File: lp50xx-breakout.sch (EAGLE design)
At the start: 17 parts, among them U1 LP5024

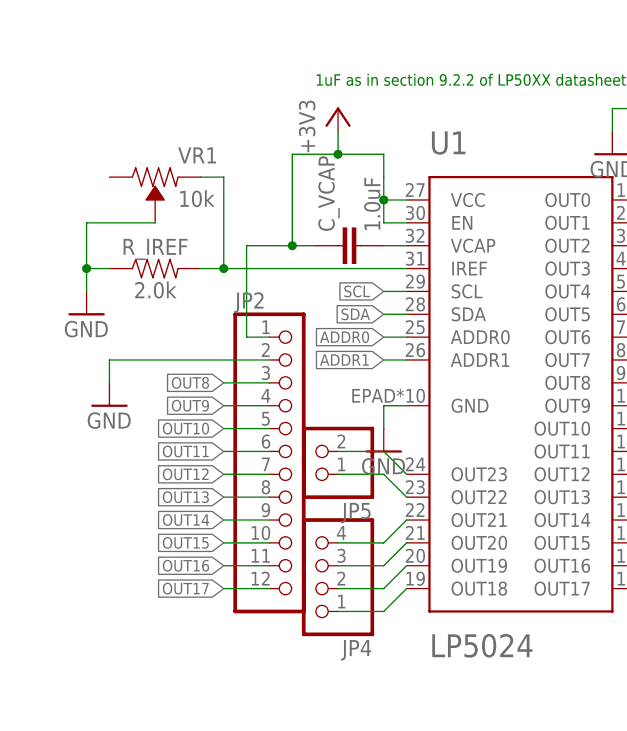
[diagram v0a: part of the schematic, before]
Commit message: Minor improvements
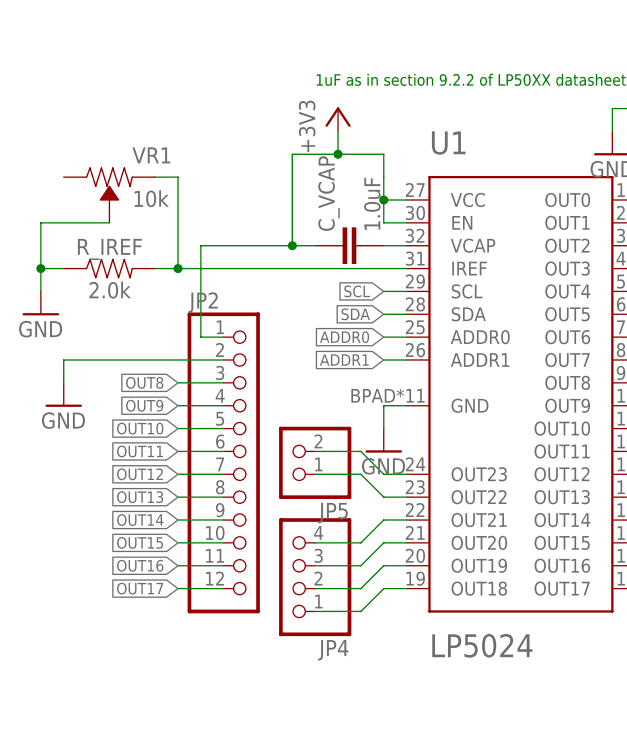
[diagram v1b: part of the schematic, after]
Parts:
- U1: device lp5018:LP5024 -> lp50xx:LP5024
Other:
- moved on the sheet: JP2, JP4, JP5, R_IREF, VR1

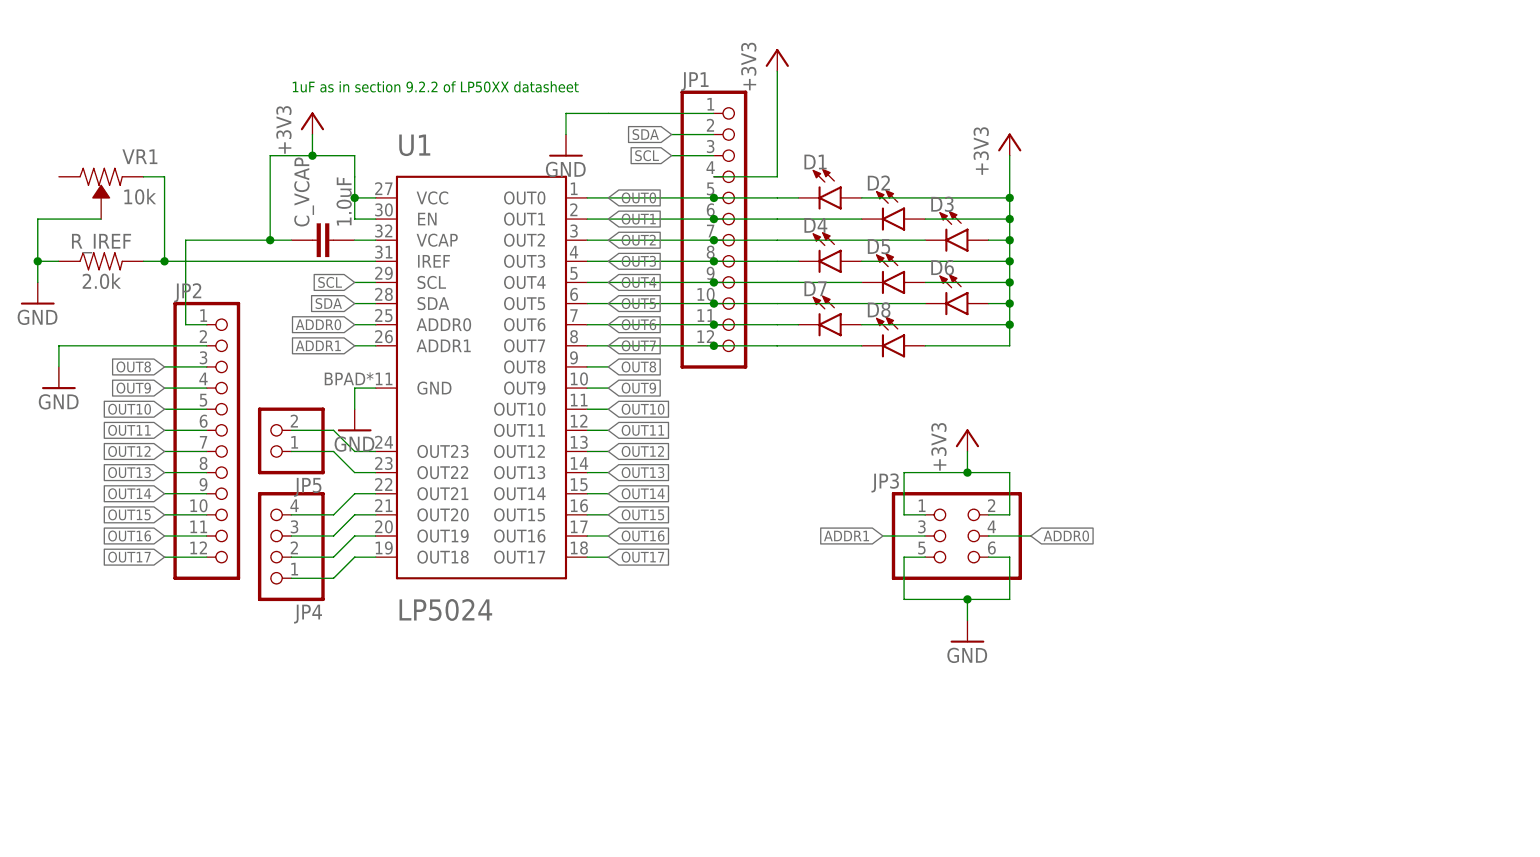
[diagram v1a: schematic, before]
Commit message: Update design
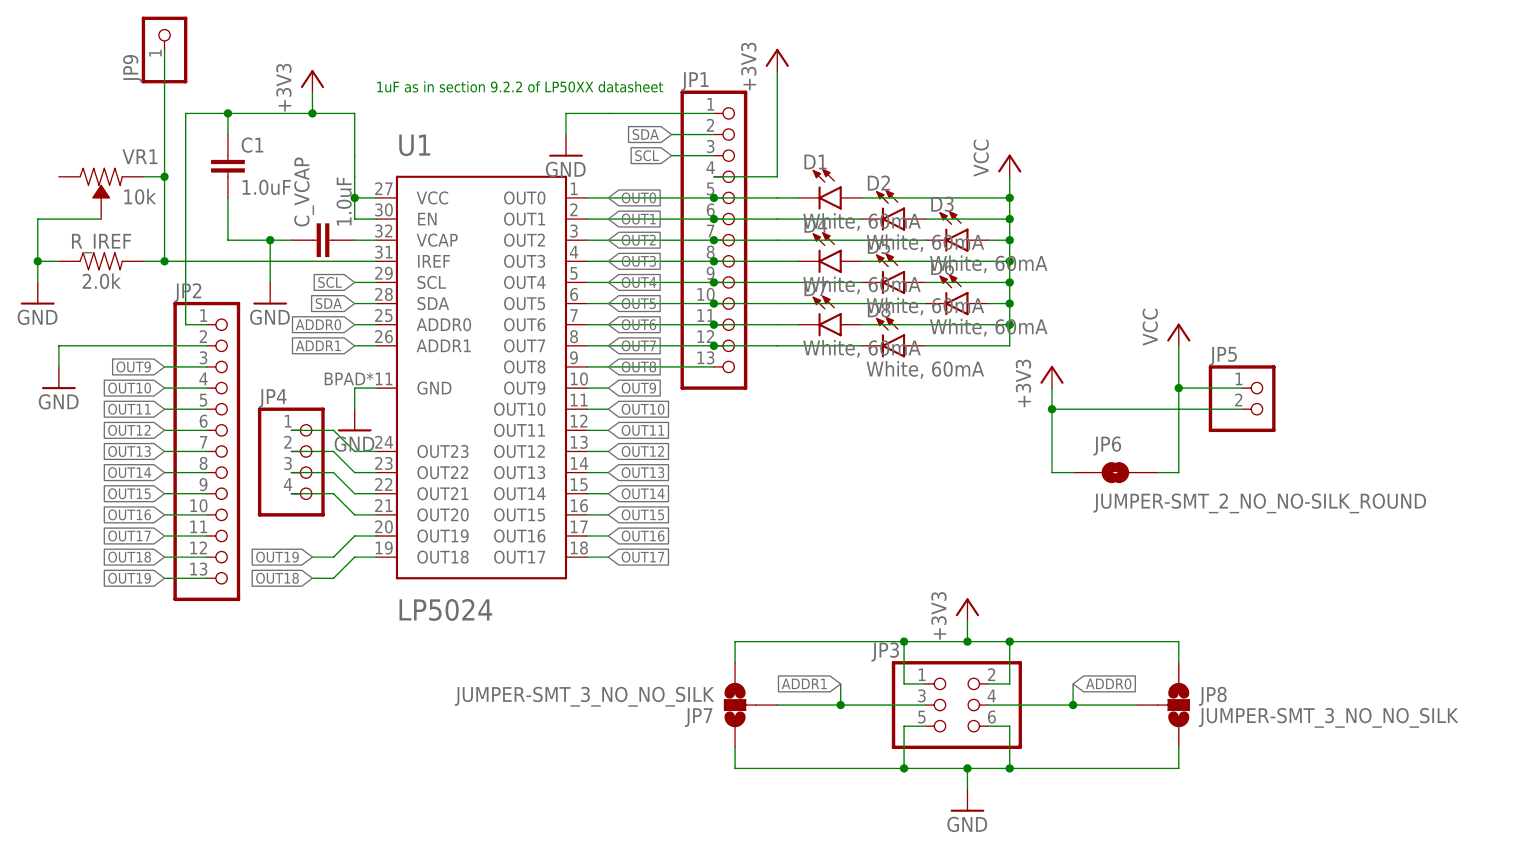
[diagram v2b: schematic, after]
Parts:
- added C1: 1.0uF, SparkFun-Capacitors:1.0UF-0603-16V-10%
- added JP6: JUMPER-SMT_2_NO_NO-SILK_ROUND, SparkFun-Jumpers:JUMPER-SMT_2_NO_NO-SILK_ROUND
- added JP7, JP8: JUMPER-SMT_3_NO_NO_SILK, SparkFun-Jumpers:JUMPER-SMT_3_NO_NO_SILK
- added JP9: (no value), pinhead-otto:PINHD-1X1
- D1, D2, D3, D4, D5, D6, D7, D8: value (none) -> White, 60mA
- JP1, JP2: device pinhead-otto:PINHD-1X12 -> pinhead-otto:PINHD-1X13
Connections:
- net N$5 renamed VCAP
- removed net N$1: R_IREF.2, U1.IREF, VR1.CCW
- new net IREF: JP9.1, R_IREF.2, U1.IREF, VR1.CCW
- new net VCC: D1.A, D2.A, D3.A, D4.A, D5.A, D6.A, D7.A, D8.A, JP5.1, JP6.2
- net +3V3: now also C1.1, JP5.2, JP6.1, JP7.3, JP8.1; no longer C_VCAP.1, D1.A, D2.A, D3.A, D4.A, D5.A, D6.A, D7.A, D8.A
- net ADDR0: now also JP8.2
- net ADDR1: now also JP7.2
- net GND: now also C1.2, C_VCAP.1, JP7.1, JP8.3
- net OUT10: now also JP2.4; no longer JP2.5
- net OUT11: now also JP2.5; no longer JP2.6
- net OUT12: now also JP2.6; no longer JP2.7
- net OUT13: now also JP2.7; no longer JP2.8
- net OUT14: now also JP2.8; no longer JP2.9
- net OUT15: now also JP2.9; no longer JP2.10
- net OUT16: now also JP2.10; no longer JP2.11
- net OUT17: now also JP2.11; no longer JP2.12
- net OUT18: now also JP2.12; no longer JP4.1
- net OUT19: now also JP2.13; no longer JP4.2
- net OUT20: now also JP4.4; no longer JP4.3
- net OUT21: now also JP4.3; no longer JP4.4
- net OUT22: now also JP4.2; no longer JP5.1
- net OUT23: now also JP4.1; no longer JP5.2
- net OUT8: now also JP1.13; no longer JP2.3
- net OUT9: now also JP2.3; no longer JP2.4
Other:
- moved on the sheet: JP3, JP4, JP5
